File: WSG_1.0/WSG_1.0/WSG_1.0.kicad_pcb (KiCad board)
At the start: 4 copper layers, 152.3 x 89.7 mm, 121 parts, among them J1 Conn_01x10, J2 USB_C_Receptacle_USB2.0_16P, J4 Conn_01x02, SW3 SW_Push, SW4 SW_Push, U1 ADS131A04IPBSR, U10 TPS22916CYFPR, U11 W25N04KVZEIR, U12 USBLC6-2SC6, U14 TPD4E1U06DBVR, U15 ESP32-S3-MINI-1U-N8, U2 DAC60501ZDGSR, U3 INA827AIDGKR, U4 INA827AIDGKR, U5 INA827AIDGKR, U6 TMP235A2DBZR, U7 BQ25180YBGR, U8 TPS63802DLAR, U9 TPS7A2025PDBVR, Y1 SiT8008AI-12-33S-16.384000

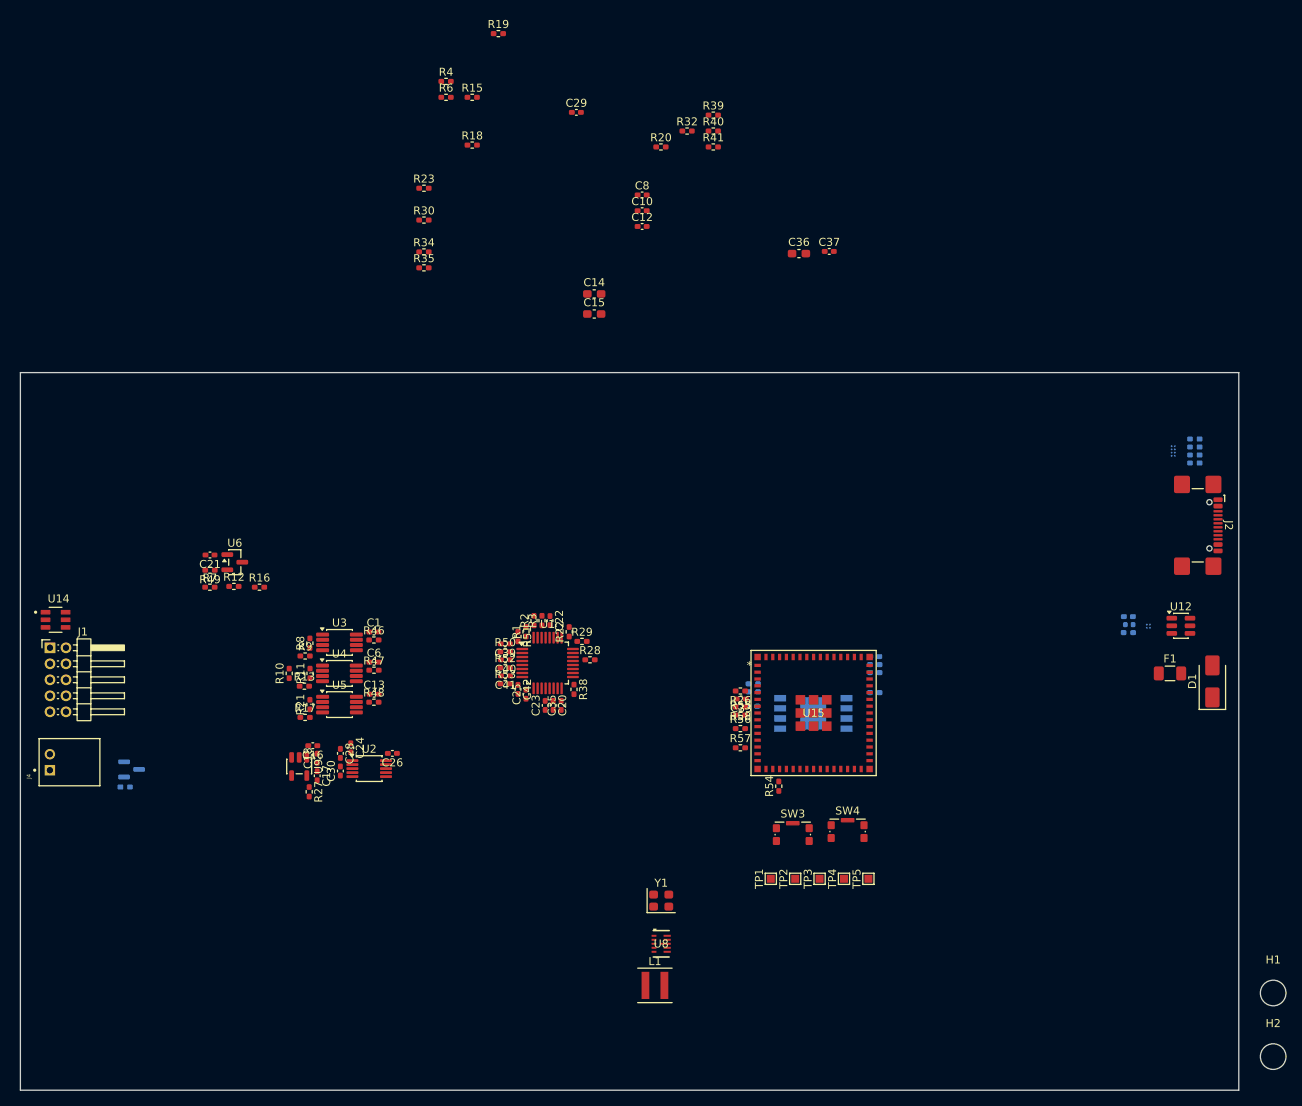
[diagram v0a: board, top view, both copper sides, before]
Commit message: new layout, trying different layout onw
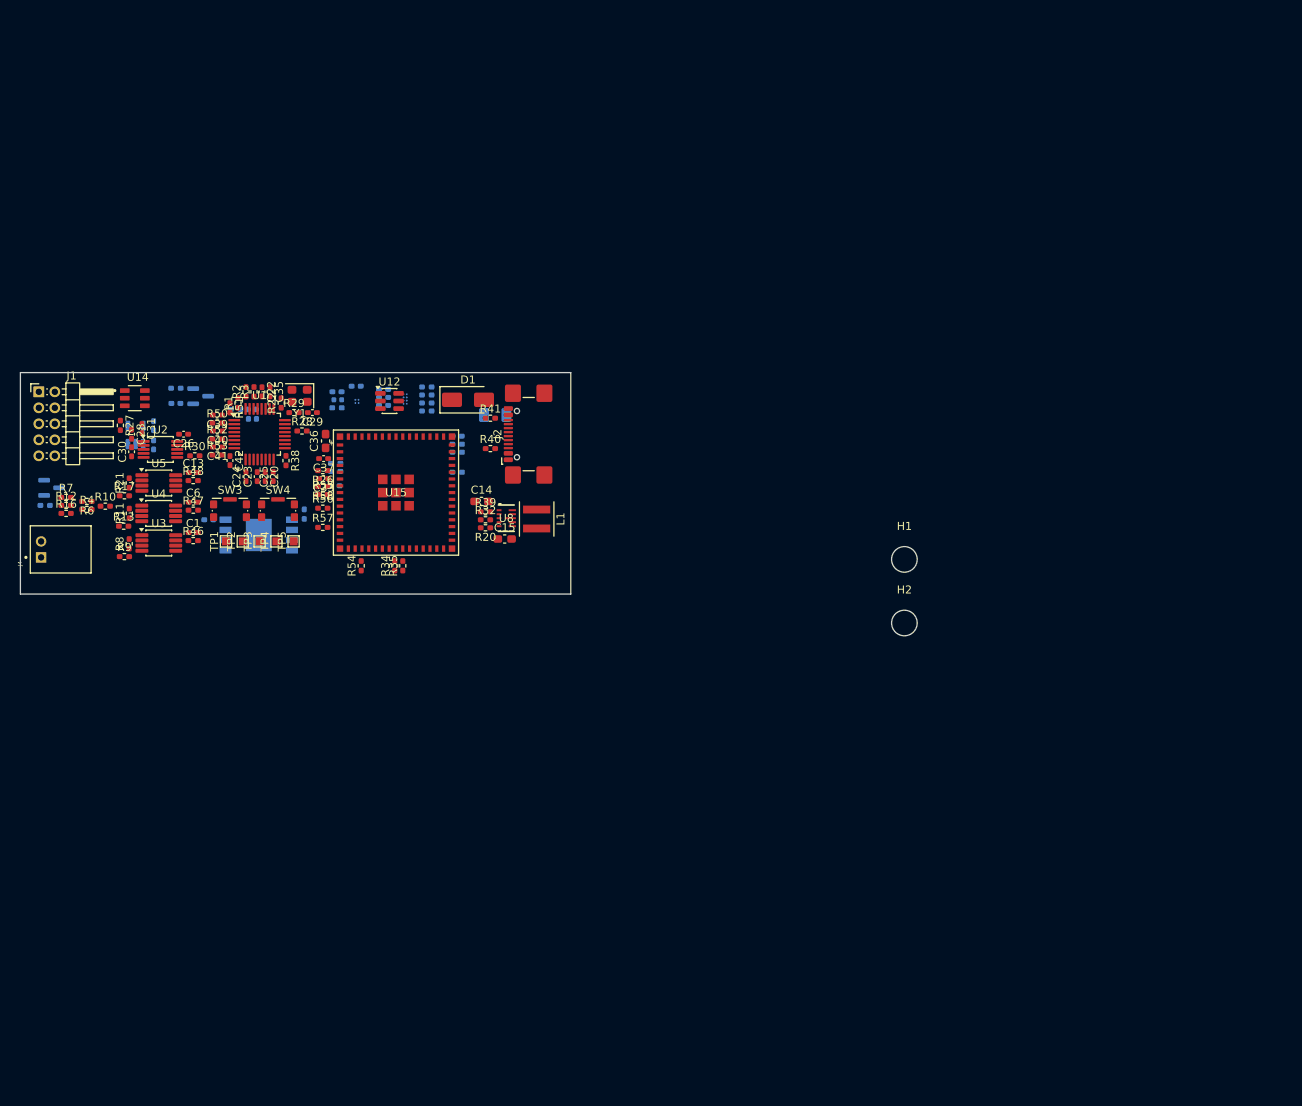
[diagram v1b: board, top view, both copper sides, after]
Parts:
- added C2: 1uF, Capacitor_SMD:C_0402_1005Metric_Pad0.74x0.62mm_HandSolder, B.Cu at (128.3, 63.1)
- added C31: 1uF, Capacitor_SMD:C_0402_1005Metric_Pad0.74x0.62mm_HandSolder, F.Cu at (101.5, 68.4)
- C10, C12, C16, C17, C18, C21, C8, F1, R15, R18, R19, R23, R49, U6, U9: moved to B.Cu
- moved C34 102.8 mm to (125.9, 63.8)
- moved FB1 102.8 mm to (126.0, 64.8)
- moved R24 102.8 mm to (125.9, 65.8)
- moved U10 102.8 mm to (128.4, 65.0)
- moved U12 102.8 mm to (132.4, 65.0)
- moved D1 99.5 mm to (142.2, 64.8), turned to 0 degrees
- moved R14 96.2 mm to (137.1, 66.2)
- moved R33 96.2 mm to (137.1, 63.2)
- moved R36 96.2 mm to (137.1, 65.2)
- moved R37 96.2 mm to (137.1, 64.2)
- moved U7 96.2 mm to (134.4, 64.7)
- moved F1 90.3 mm to (145.7, 66.7), turned to 180 degrees
- moved TP5 83.3 mm to (120.5, 82.5)
- moved TP4 82.5 mm to (118.3, 82.5)
- moved J2 82.1 mm to (151.0, 69.1), turned to 90 degrees
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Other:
- board size 152.3 x 89.7 mm -> 68.8 x 27.7 mm
